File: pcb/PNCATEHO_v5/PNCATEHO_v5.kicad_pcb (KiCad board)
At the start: 2 copper layers, 97 x 59 mm, 27 parts, among them J1 TestPoint_2Pole, SW1 SW_PUSH, SW10 SW_PUSH, SW2 SW_PUSH, SW3 SW_PUSH, SW4 SW_PUSH, SW5 SW_PUSH, SW6 SW_PUSH, SW7 SW_PUSH, SW8 SW_PUSH, SW9 SW_PUSH, U1 ProMicro_r

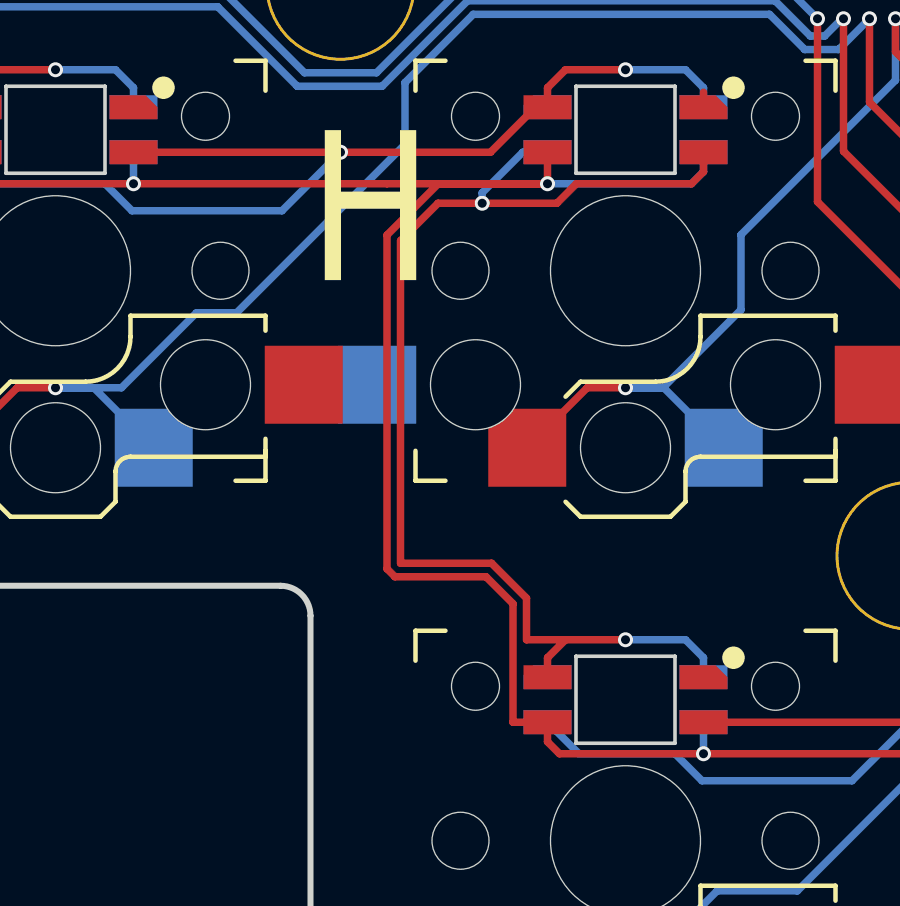
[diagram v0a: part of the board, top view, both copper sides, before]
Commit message: Small beauty fix
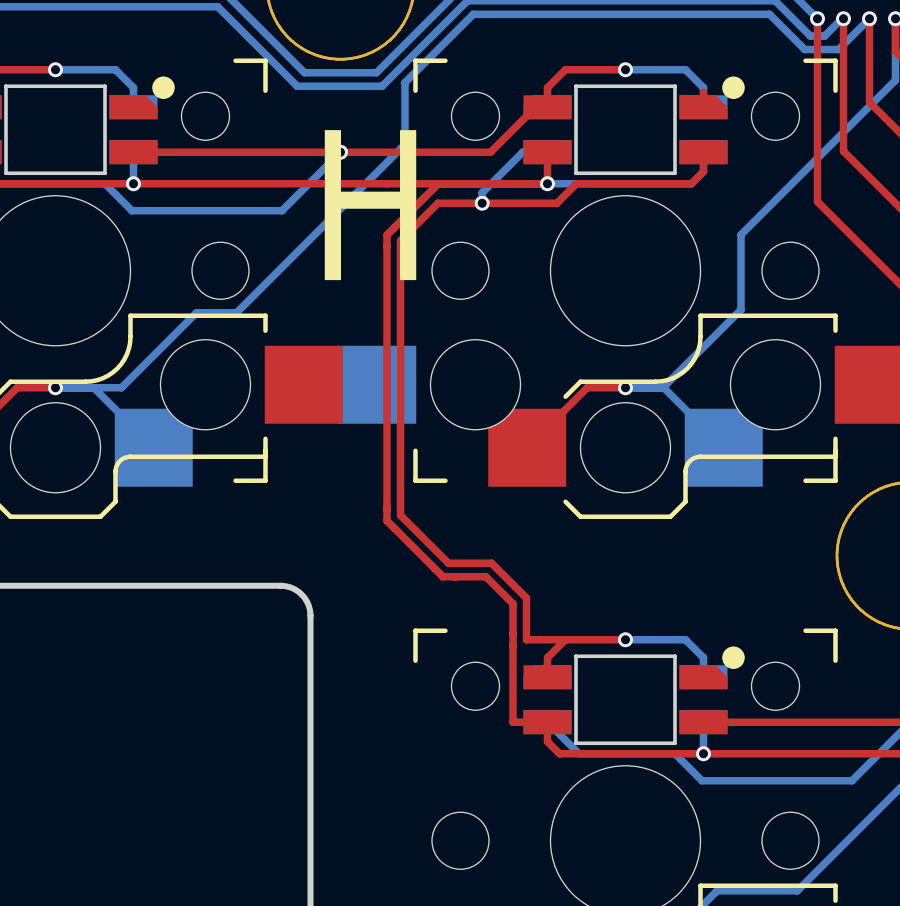
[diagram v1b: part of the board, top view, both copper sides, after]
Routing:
- net Net-(LED2-DOUT): track 39.9 -> 39.0 mm
- net VCC: track 254.2 -> 253.2 mm
